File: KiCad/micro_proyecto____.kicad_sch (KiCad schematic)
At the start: 33 parts, among them J1 Conn_01x05, J2 Conn_01x02, J3 Conn_01x02, J4 Conn_01x02, J5 Conn_01x02, SW1 SW_Push, SW2 SW_SPST, SW3 SW_SPST, SW4 SW_SPST, SW5 SW_SPST, U1 PIC24HJ128GP502, Y1 Crystal

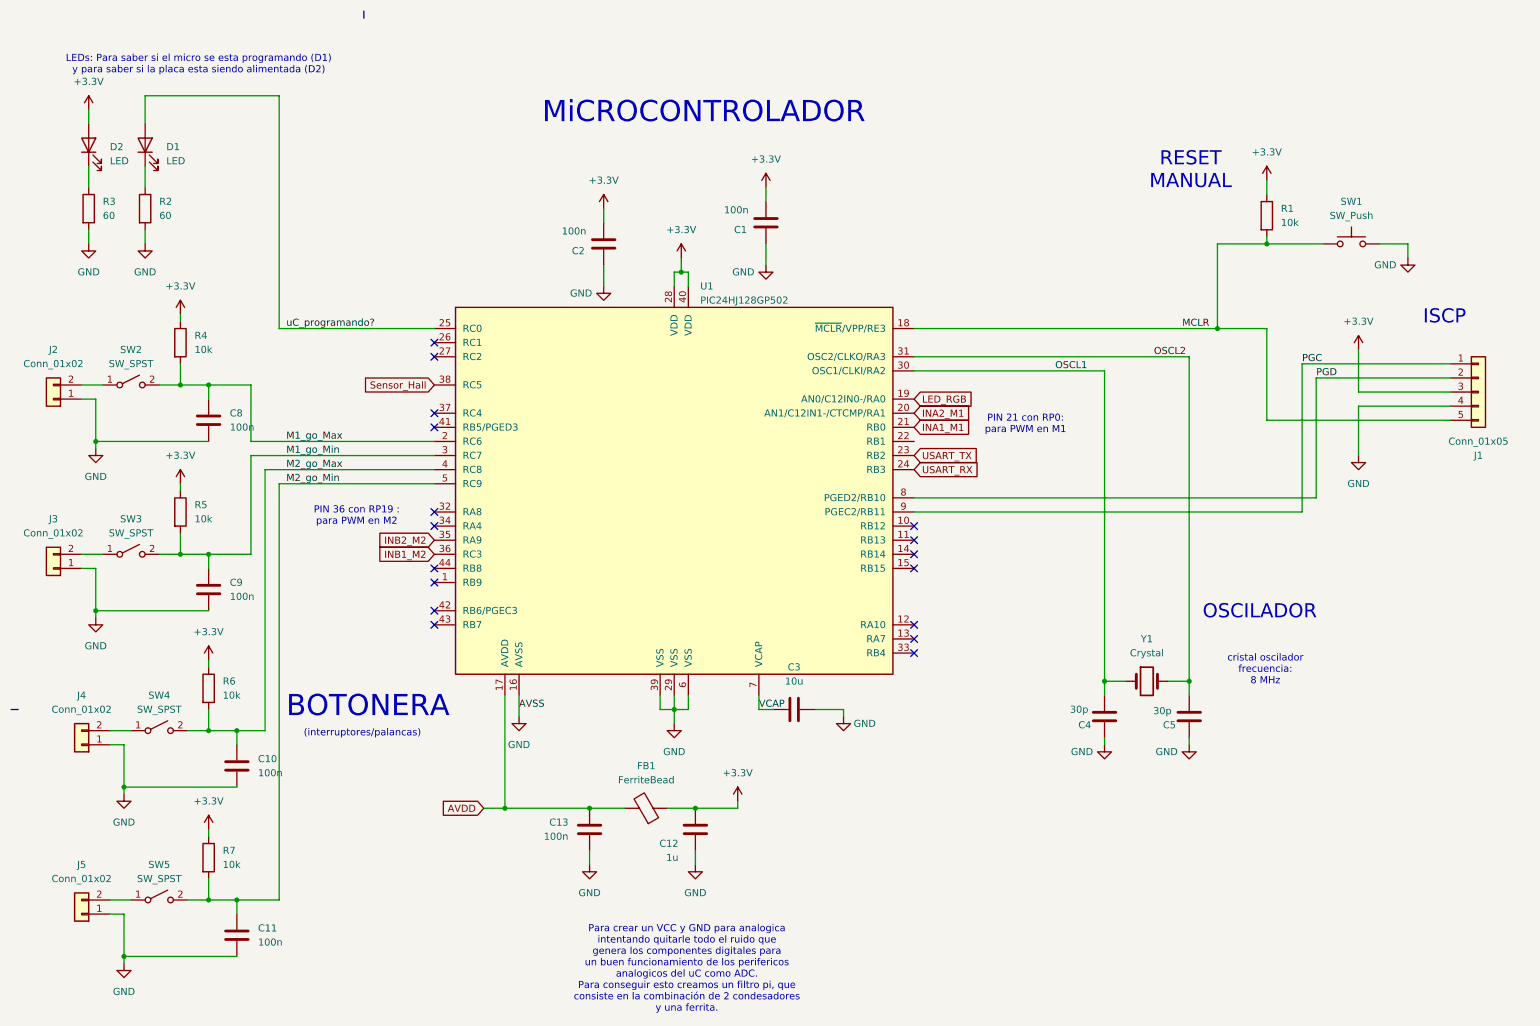
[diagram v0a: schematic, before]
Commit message: Nuevos cambios esquemativo v3
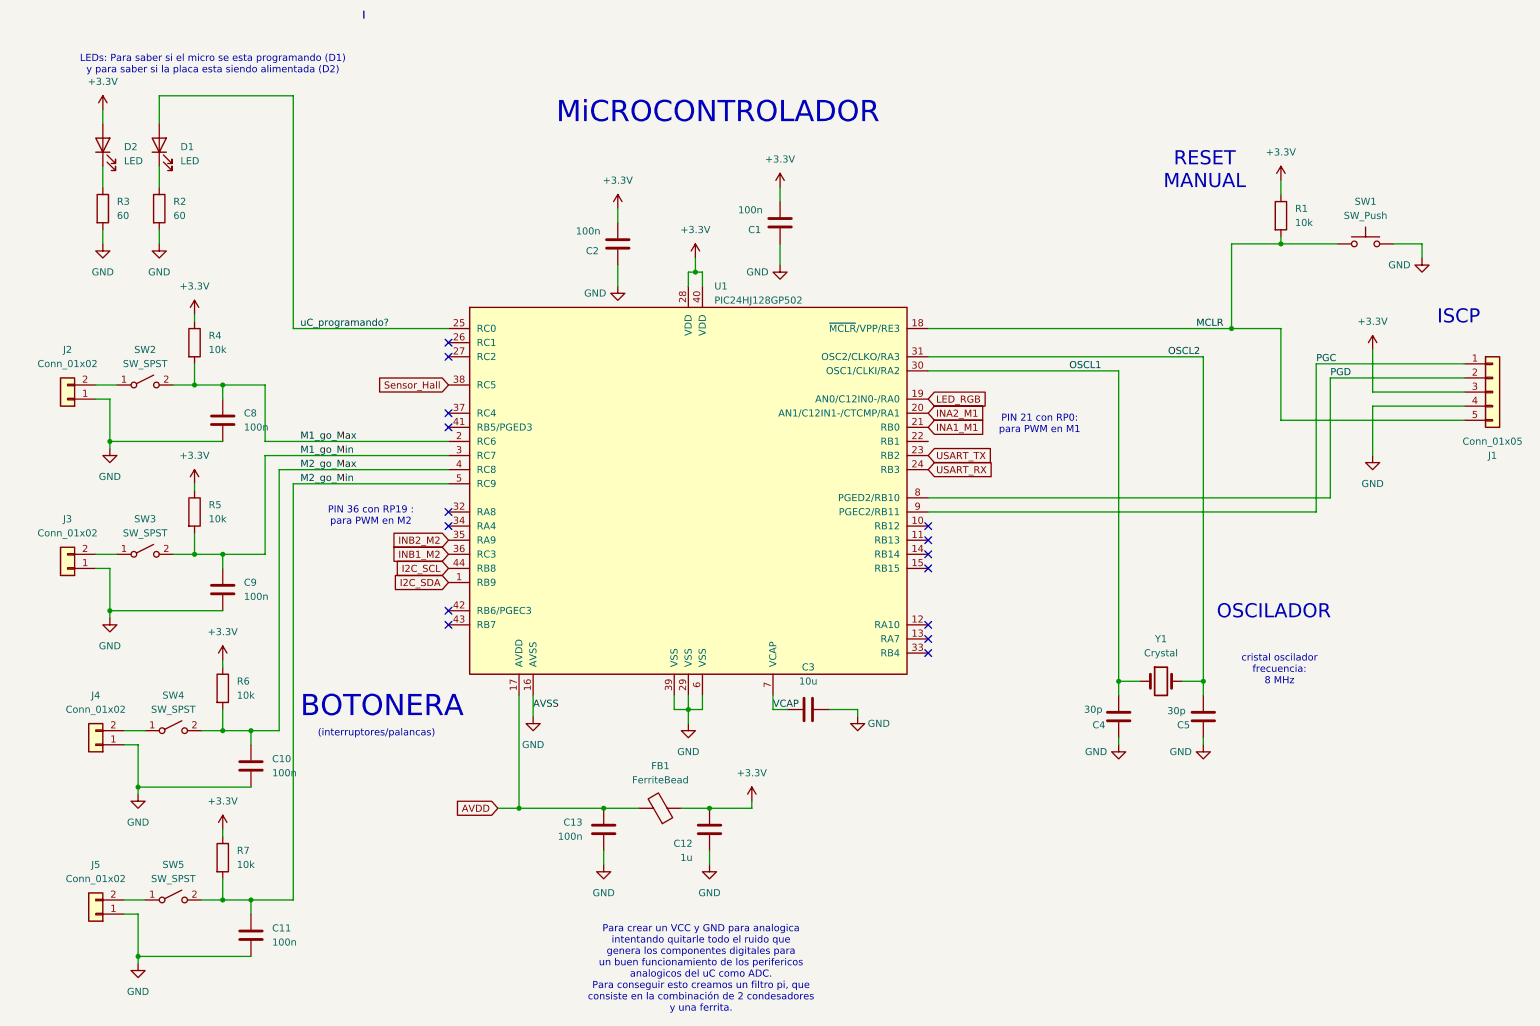
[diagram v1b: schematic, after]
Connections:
- net I2C_SDA: now reaches U1.1 (RB9)
- net I2C_SCL: now reaches U1.44 (RB8)
- no-connect marks 17 -> 15
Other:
- moved on the sheet: C1, C10, C11, C12, C13, C2, C3, C4, C5, C8, C9, D1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
